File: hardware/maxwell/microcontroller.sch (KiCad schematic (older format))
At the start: 16 parts, among them U7 STM32F103RETx, Y2 8M, Y3 32.768k

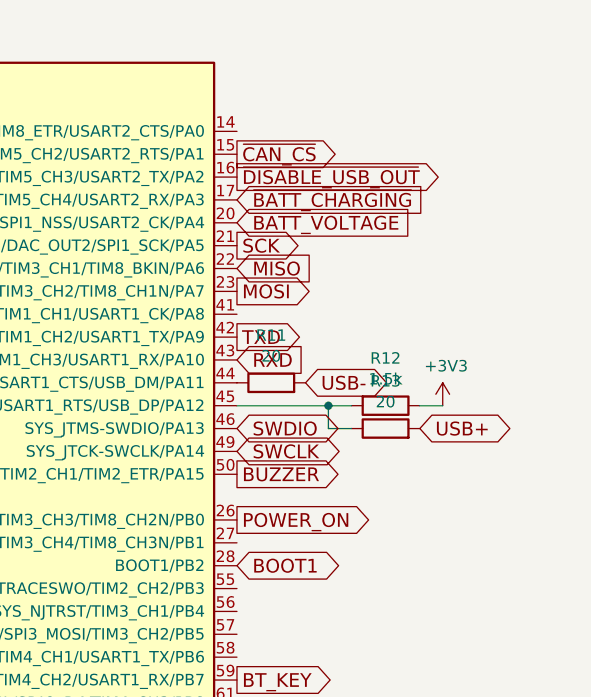
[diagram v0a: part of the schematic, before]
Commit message: More minor changes and fixes.
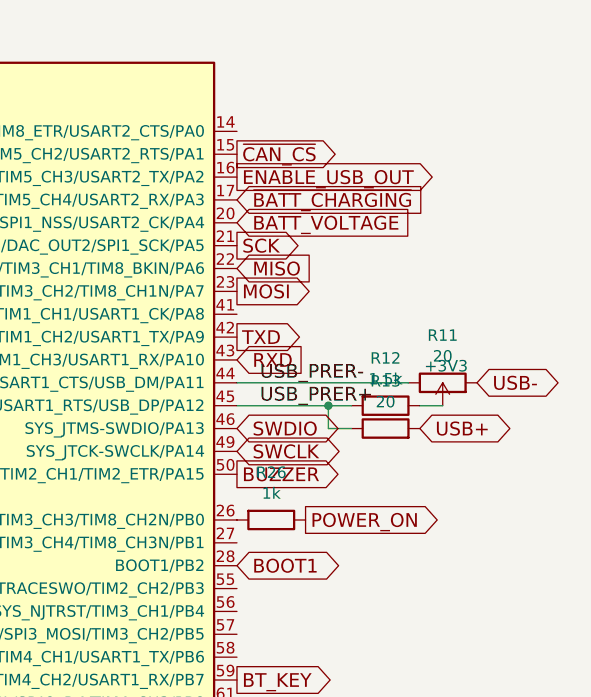
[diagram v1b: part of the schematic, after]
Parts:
- added R26: 1k, coddingtonbear/coddingtonbear.pretty:0805_Milling, symbol R
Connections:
- net POWER_ON: now also R26.1; no longer U7.26 (ADC1_IN8/ADC2_IN8/TIM1_CH2N/TIM3_CH3/TIM8_CH2N/PB0)
- net USB_PRER-: now reaches R11.1, U7.44 (ADC1_EXTI11/ADC2_EXTI11/CAN_RX/TIM1_CH4/USART1_CTS/USB_DM/PA11)
- net USB_PRER+: now reaches R12.2, R13.1, U7.45 (CAN_TX/TIM1_ETR/USART1_RTS/USB_DP/PA12)
- net ~DISABLE_USB_OUT renamed ENABLE_USB_OUT
- new net: R26.2, U7.26 (ADC1_IN8/ADC2_IN8/TIM1_CH2N/TIM3_CH3/TIM8_CH2N/PB0)
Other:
- moved on the sheet: R11
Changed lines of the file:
@@
 	8900 3550 8900 3450
 Connection ~ 8900 3450
-Text GLabel 8800 3350 2    60   BiDi ~ 0
+Text GLabel 9550 3350 2    60   BiDi ~ 0
 USB-
 $Comp
@@
 L R R11
 U 1 1 5A1FCF7E
-P 8650 3350
-F 0 "R11" V 8857 3350 50  0000 C CNN
-F 1 "20" V 8766 3350 50  0000 C CNN
-F 2 "coddingtonbear/coddingtonbear.pretty:0805_Milling" V 8580 3350 50  0001 C CNN
-F 3 "" H 8650 3350 50  0001 C CNN
-	1    8650 3350
+P 9400 3350
+F 0 "R11" V 9607 3350 50  0000 C CNN
+F 1 "20" V 9516 3350 50  0000 C CNN
+F 2 "coddingtonbear/coddingtonbear.pretty:0805_Milling" V 9330 3350 50  0001 C CNN
+F 3 "" H 9400 3350 50  0001 C CNN
+	1    9400 3350
 	0    -1   -1   0
 $EndComp
@@
 SPEED
 Text GLabel 8500 2450 2    60   Output ~ 0
-~DISABLE_USB_OUT
+ENABLE_USB_OUT
 Text GLabel 8500 2550 2    60   Input ~ 0
 ~BATT_CHARGING
-Text GLabel 8500 3950 2    60   Output ~ 0
+Text GLabel 8800 3950 2    60   Output ~ 0
 POWER_ON
 Text GLabel 8500 2750 2    60   Output ~ 0
@@
 Text GLabel 8500 4850 2    60   Output ~ 0
 ENABLE_BATT_POWER
+$Comp
+L R R26
+U 1 1 5A260AAF
+P 8650 3950
+F 0 "R26" V 8443 3950 50  0000 C CNN
+F 1 "1k" V 8534 3950 50  0000 C CNN
+F 2 "coddingtonbear/coddingtonbear.pretty:0805_Milling" V 8580 3950 50  0001 C CNN
+F 3 "" H 8650 3950 50  0001 C CNN
+	1    8650 3950
+	0    1    1    0
+$EndComp
+Wire Wire Line
+	8500 3350 9250 3350
+Text Label 8600 3350 0    60   ~ 0
+USB_PRER-
+Text Label 8600 3450 0    60   ~ 0
+USB_PRER+
 $EndSCHEMATC

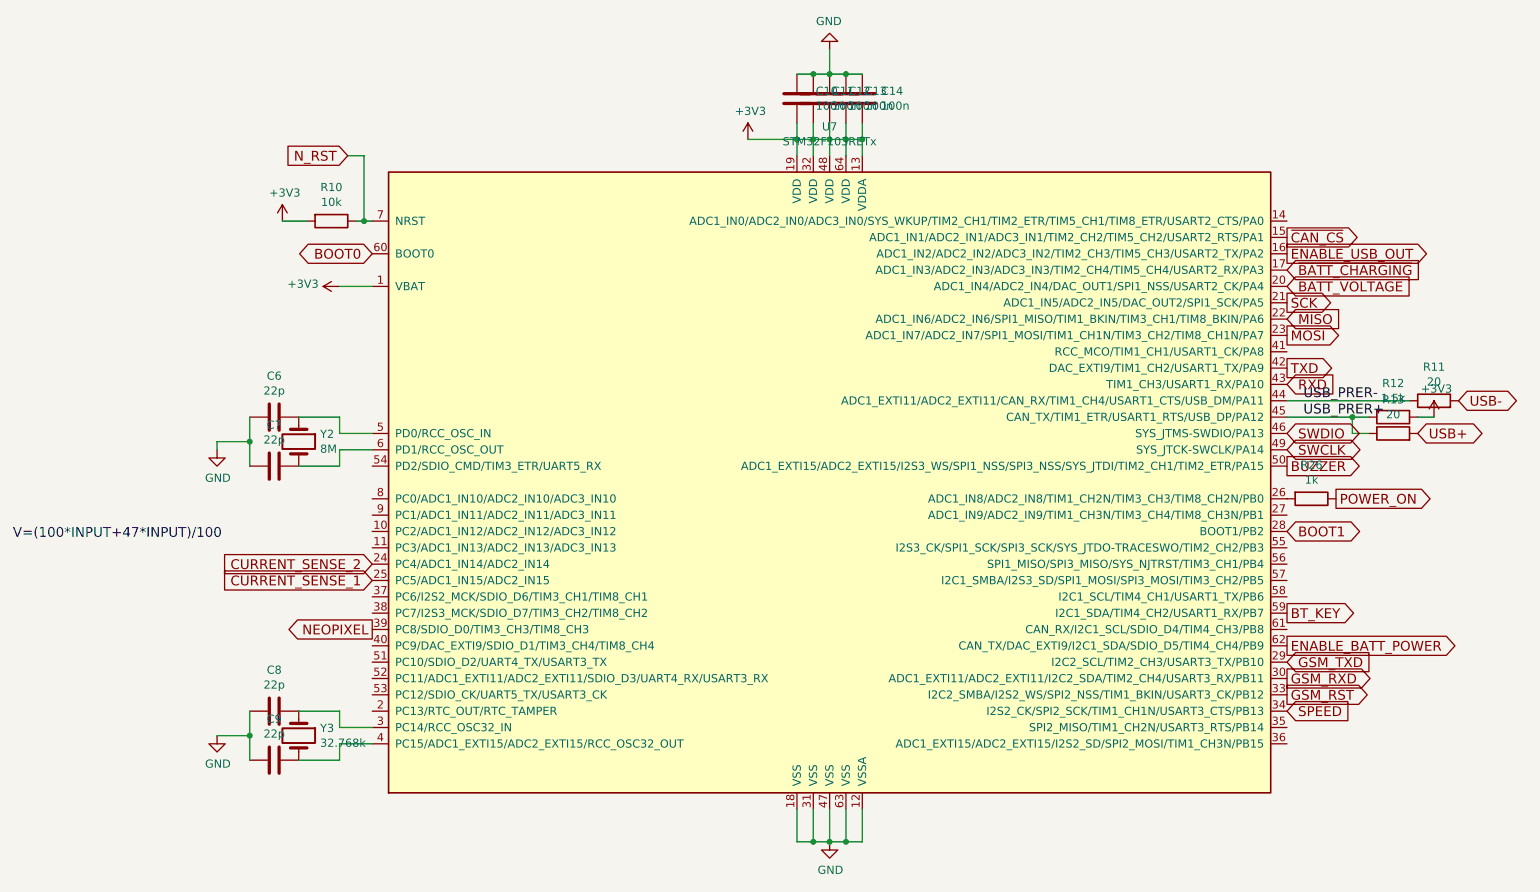
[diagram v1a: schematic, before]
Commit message: More fixes, additions, improvements.
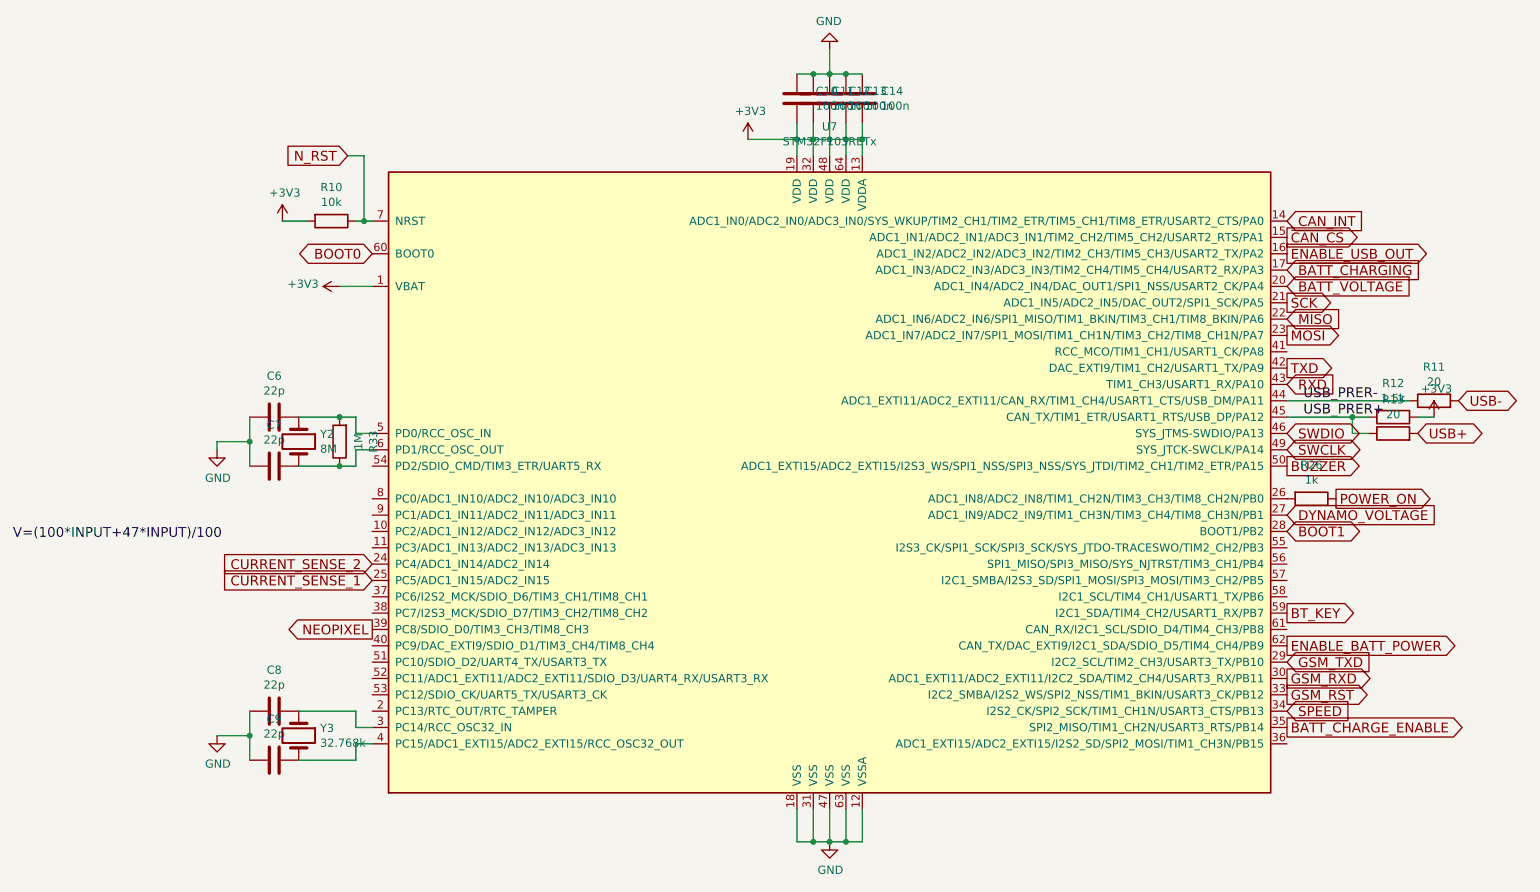
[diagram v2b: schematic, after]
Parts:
- added R33: 1M, coddingtonbear/coddingtonbear.pretty:0805_Milling, symbol R
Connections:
- net CAN_INT: now reaches U7.14 (ADC1_IN0/ADC2_IN0/ADC3_IN0/SYS_WKUP/TIM2_CH1/TIM2_ETR/TIM5_CH1/TIM8_ETR/USART2_CTS/PA0)
- net DYNAMO_VOLTAGE: now reaches U7.27 (ADC1_IN9/ADC2_IN9/TIM1_CH3N/TIM3_CH4/TIM8_CH3N/PB1)
- net BATT_CHARGE_ENABLE: now reaches U7.35 (SPI2_MISO/TIM1_CH2N/USART3_RTS/PB14)
- net at C6.1, U7.5 (PD0/RCC_OSC_IN), Y2.1: now also R33.2
- net at C7.1, U7.6 (PD1/RCC_OSC_OUT), Y2.2: now also R33.1
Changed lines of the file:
@@
 	1950 3600 2150 3600
 Connection ~ 2150 3600
-Wire Wire Line
-	2450 3450 2700 3450
-Wire Wire Line
-	2700 3450 2700 3550
-Wire Wire Line
-	2700 3550 2900 3550
-Wire Wire Line
-	2450 3750 2700 3750
-Wire Wire Line
-	2700 3750 2700 3650
-Wire Wire Line
-	2700 3650 2900 3650
 $Comp
 L Crystal Y3
@@
 	1    0    0    -1
 $EndComp
-Wire Wire Line
-	2450 5250 2700 5250
-Wire Wire Line
-	2700 5250 2700 5350
-Wire Wire Line
-	2700 5350 2900 5350
-Wire Wire Line
-	2450 5550 2700 5550
-Wire Wire Line
-	2700 5550 2700 5450
-Wire Wire Line
-	2700 5450 2900 5450
 Wire Wire Line
 	2150 5250 2150 5550
@@
 Text Label 8600 3450 0    60   ~ 0
 USB_PRER+
+Text GLabel 8500 2250 2    60   Input ~ 0
+CAN_INT
+$Comp
+L R R33
+U 1 1 5A2732F7
+P 2700 3600
+F 0 "R33" V 2493 3600 50  0000 C CNN
+F 1 "1M" V 2584 3600 50  0000 C CNN
+F 2 "coddingtonbear/coddingtonbear.pretty:0805_Milling" V 2630 3600 50  0001 C CNN
+F 3 "" H 2700 3600 50  0001 C CNN
+	1    2700 3600
+	-1   0    0    1
+$EndComp
+Wire Wire Line
+	2450 5250 2800 5250
+Wire Wire Line
+	2800 5250 2800 5350
+Wire Wire Line
+	2800 5350 2900 5350
+Wire Wire Line
+	2900 5450 2800 5450
+Wire Wire Line
+	2800 5450 2800 5550
+Wire Wire Line
+	2800 5550 2450 5550
+Wire Wire Line
+	2450 3450 2800 3450
+Wire Wire Line
+	2800 3450 2800 3550
+Wire Wire Line
+	2800 3550 2900 3550
+Connection ~ 2700 3450
+Wire Wire Line
+	2450 3750 2800 3750
+Wire Wire Line
+	2800 3750 2800 3650
+Wire Wire Line
+	2800 3650 2900 3650
+Connection ~ 2700 3750
+Text GLabel 8500 4050 2    60   Input ~ 0
+DYNAMO_VOLTAGE
+Text GLabel 8500 5350 2    60   Output ~ 0
+BATT_CHARGE_ENABLE
 $EndSCHEMATC

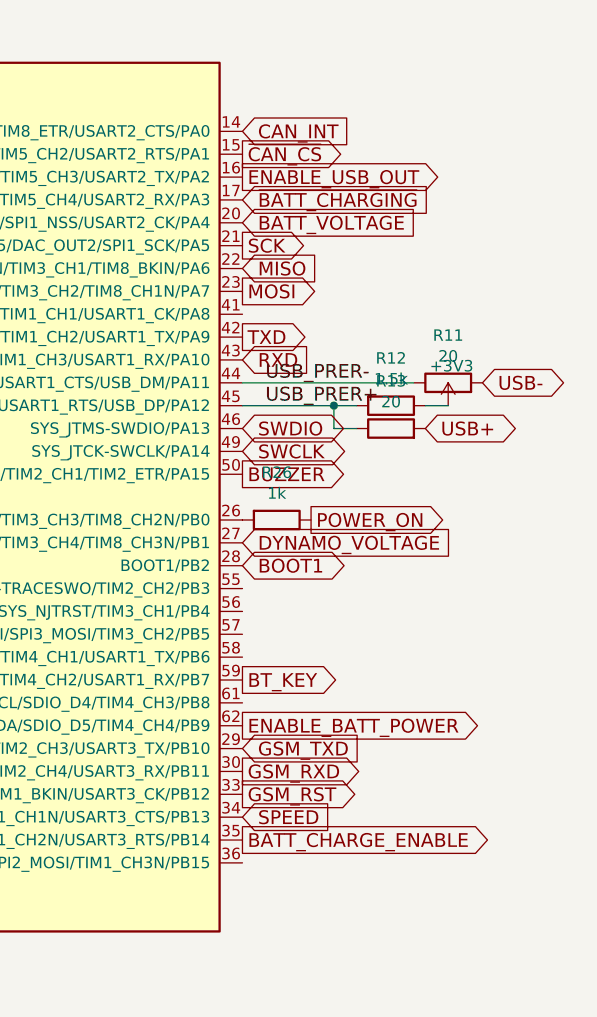
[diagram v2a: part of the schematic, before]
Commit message: Fixed just...an unbelievable number of bugs.
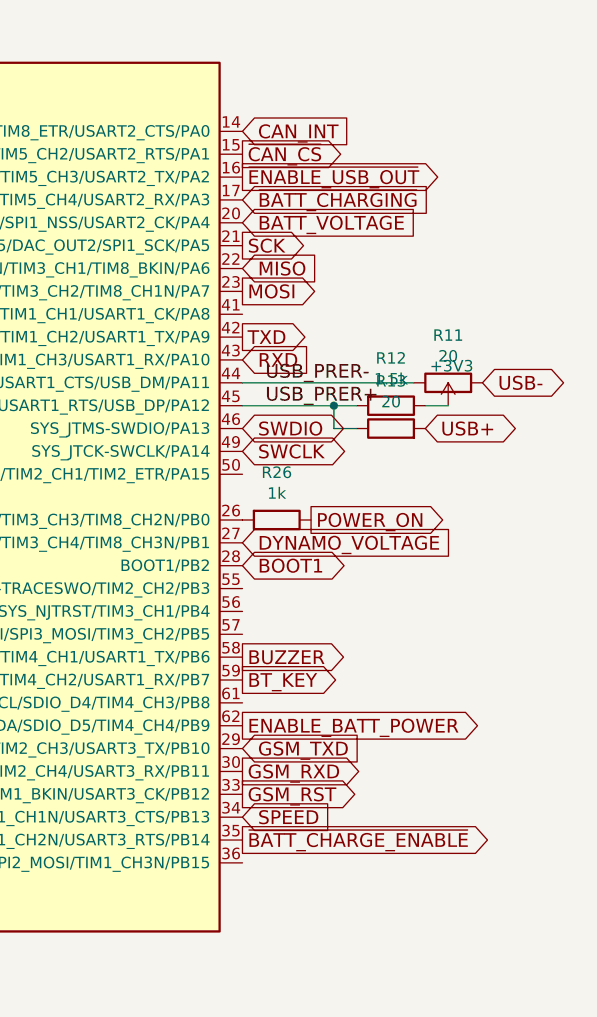
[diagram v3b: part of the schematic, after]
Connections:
- net BUZZER: now also U7.58 (I2C1_SCL/TIM4_CH1/USART1_TX/PB6); no longer U7.50 (ADC1_EXTI15/ADC2_EXTI15/I2S3_WS/SPI1_NSS/SPI3_NSS/SYS_JTDI/TIM2_CH1/TIM2_ETR/PA15)
- net BATT_CHARGE_ENABLE renamed ~BATT_CHARGE_ENABLE
- net ENABLE_USB_OUT renamed ~ENABLE_USB_OUT
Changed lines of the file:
@@
 SPEED
 Text GLabel 8500 2450 2    60   Output ~ 0
-ENABLE_USB_OUT
+~ENABLE_USB_OUT
 Text GLabel 8500 2550 2    60   Input ~ 0
 ~BATT_CHARGING
@@
 Text Notes 700  4200 0    60   ~ 0
 V=(100*INPUT+47*INPUT)/100
-Text GLabel 8500 3750 2    60   Output ~ 0
+Text GLabel 8500 4550 2    60   Output ~ 0
 BUZZER
 Text GLabel 2900 4750 0    60   Output ~ 0
@@
 DYNAMO_VOLTAGE
 Text GLabel 8500 5350 2    60   Output ~ 0
-BATT_CHARGE_ENABLE
+~BATT_CHARGE_ENABLE
 $EndSCHEMATC
